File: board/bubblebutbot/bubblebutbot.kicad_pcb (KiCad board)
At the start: 2 copper layers, 66.5 x 28.4 mm, 59 parts, among them J1 JST XH, J10 JST XH, J13 JST XH, J2 USB_C_Receptacle, J3 Conn_01x03_Socket, J4 Conn_01x03_Socket, J7 Conn_01x03_Socket, SW1 SW_Push, SW2 SW_Push, U1 DRV8833PWP, U2 ESP32-S3-WROOM-1, U3 AP63203WU, U4 LIS3DH

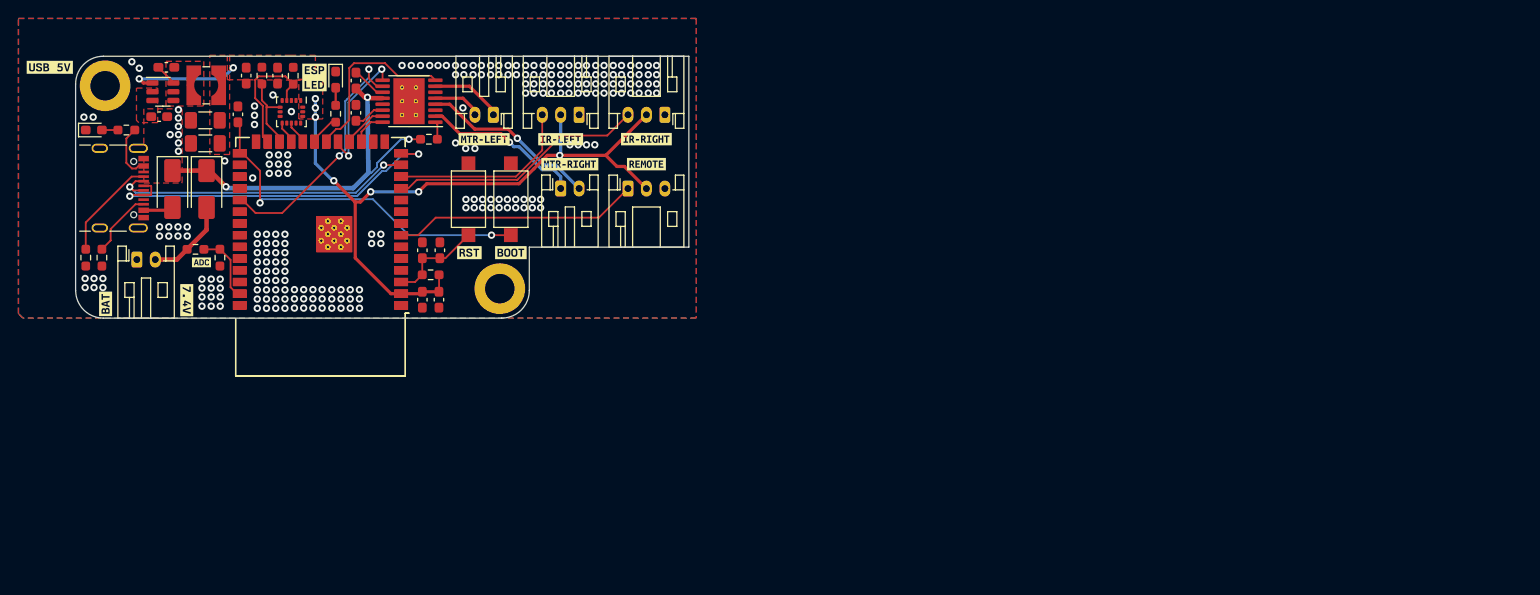
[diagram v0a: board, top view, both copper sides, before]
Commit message: prod 1v7
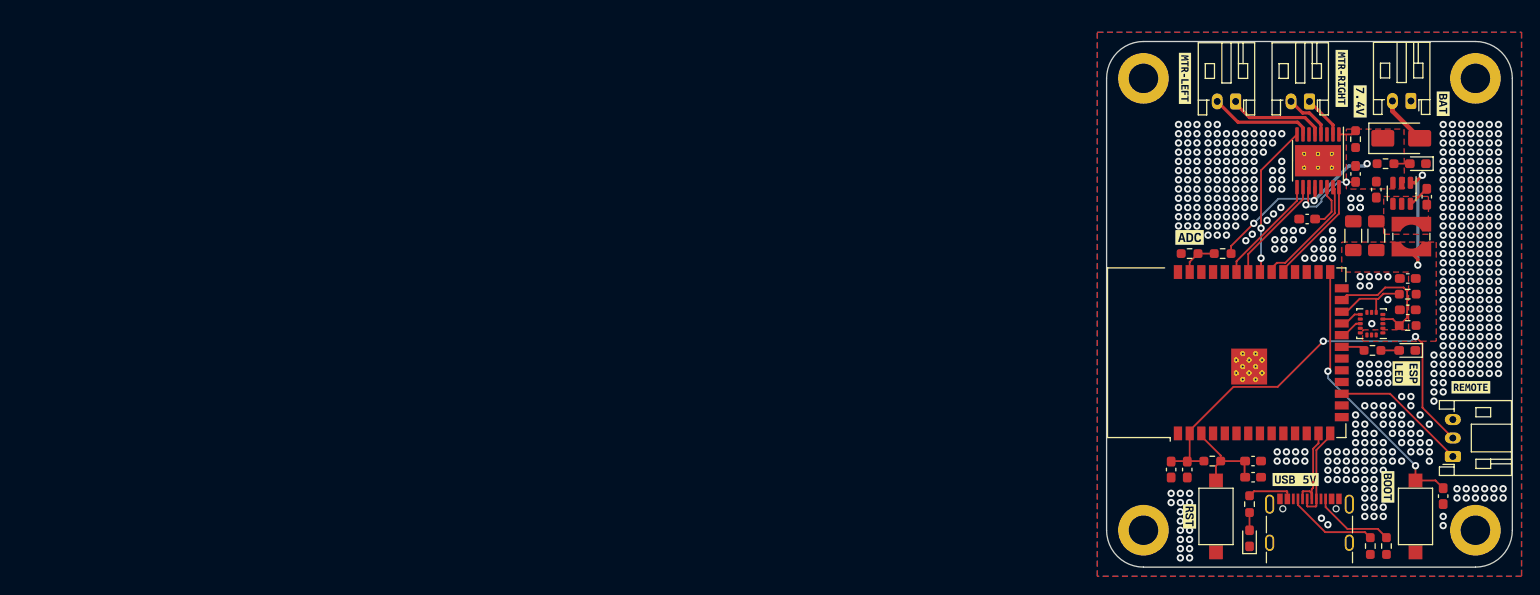
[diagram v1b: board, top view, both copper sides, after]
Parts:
- removed J3, J4: Conn_01x03_Socket, Connector_JST:JST_PH_S3B-PH-K_1x03_P2.00mm_Horizontal
- removed the U2 at (97.8, 47.4)
- removed kibuzzard-656B6BB3: G***, kibuzzard-656B6BB3
- removed kibuzzard-65B534D1: G***, kibuzzard-65B534D1
- removed kibuzzard-65B534EC: G***, kibuzzard-65B534EC
- removed kibuzzard-65B53FA4: G***, kibuzzard-65B53FA4
- added H3: MountingHole, MountingHole:MountingHole_3.2mm_M3_ISO14580_Pad, F.Cu at (223.0, 77.0)
- added H4: MountingHole, MountingHole:MountingHole_3.2mm_M3_ISO14580_Pad, F.Cu at (187.0, 28.0)
- added R3: 5.1K, Resistor_SMD:R_0603_1608Metric_Pad0.98x0.95mm_HandSolder, F.Cu at (213.2, 37.2)
- added kibuzzard-65BE7DA5: G***, kibuzzard-65BE7DA5, F.Cu at (192.0, 45.2)
- added kibuzzard-65BE89A1: G***, kibuzzard-65BE89A1, B.Cu at (205.8, 59.5)
- D2: value SS14 -> LED; footprint Diode_SMD:D_SMA -> LED_SMD:LED_0603_1608Metric_Pad1.05x0.95mm_HandSolder
- moved kibuzzard-65B53096 146.7 mm to (219.5, 30.8), turned to -90 degrees
- moved R4 142.8 mm to (211.6, 78.7)
- moved R7 142.8 mm to (213.3, 78.7)
- moved kibuzzard-65B52192 142.3 mm to (203.5, 71.5)
- moved J1 139.2 mm to (216.0, 30.4), turned to 180 degrees
- moved C11 137.4 mm to (217.7, 40.8), turned to 90 degrees
- moved C14 137.1 mm to (219.5, 73.3), turned to -90 degrees
- moved J2 135.4 mm to (205.0, 77.3), turned to 0 degrees
- moved D2 135.1 mm to (216.8, 37.2), turned to 180 degrees
- moved U3 134.8 mm to (215.0, 40.5), turned to -90 degrees
- moved D3 132.9 mm to (198.5, 77.9), turned to 90 degrees
- moved C9 132.2 mm to (212.2, 40.1), turned to -90 degrees
- moved L1 131.7 mm to (216.1, 45.2), turned to 0 degrees
- moved D4 129.7 mm to (214.9, 34.5), turned to 0 degrees
- moved kibuzzard-65B53DEB 129.1 mm to (210.5, 30.5)
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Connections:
- net MOTOR-RIGHT-FL renamed MOTOR-RIGHT-A
- net MOTOR-RIGHT-FR renamed MOTOR-RIGHT-B
- D2 pad 1: BAT_OUT -> GND
- D2 pad 2: 5V_USB_POWER -> Net-(D2-A)
- J10 pad 1: MOTOR-LEFT-FL -> MOTOR-LEFT-A
- J10 pad 2: MOTOR-LEFT-FR -> MOTOR-LEFT-B
- R6 pad 2: +7.5V -> BAT_OUT
- U1 pad 5: MOTOR-LEFT-FR -> MOTOR-LEFT-A
- U1 pad 7: MOTOR-LEFT-FL -> MOTOR-LEFT-B
- U2 pad 10: ESP32-SRV-F -> unconnected-(U2-GPIO17/U1TXD/ADC2_CH6-Pad10)
- U2 pad 11: ESP32-IR-FR -> unconnected-(U2-GPIO18/U1RXD/ADC2_CH7/CLK_OUT3-Pad11)
- U2 pad 12: ESP32-IR-FL -> unconnected-(U2-GPIO8/TOUCH8/ADC1_CH7/SUBSPICS1-Pad12)
- U2 pad 17: ESP32-MOTOR-AIN1 -> ESP32-REMOTE
- U2 pad 18: ESP32-MOTOR-AIN2 -> unconnected-(U2-GPIO10/TOUCH10/ADC1_CH9/FSPICS0/FSPIIO4/SUBSPICS0-Pad18)
- U2 pad 19: ESP32-MOTOR-BIN1 -> unconnected-(U2-GPIO11/TOUCH11/ADC2_CH0/FSPID/FSPIIO5/SUBSPID-Pad19)
- U2 pad 20: ESP32-MOTOR-FAULT -> unconnected-(U2-GPIO12/TOUCH12/ADC2_CH1/FSPICLK/FSPIIO6/SUBSPICLK-Pad20)
- U2 pad 31: ESP32-MOTOR-BIN2 -> ESP32-MOTOR-AIN1
- U2 pad 32: unconnected-(U2-MTCK/GPIO39/CLK_OUT3/SUBSPICS1-Pad32) -> ESP32-MOTOR-AIN2
- U2 pad 33: unconnected-(U2-MTDO/GPIO40/CLK_OUT2-Pad33) -> ESP32-MOTOR-FAULT
- U2 pad 34: unconnected-(U2-MTDI/GPIO41/CLK_OUT1-Pad34) -> ESP32-MOTOR-BIN2
- U2 pad 35: unconnected-(U2-MTMS/GPIO42-Pad35) -> ESP32-MOTOR-BIN1
- U2 pad 5: ESP32-LF-RIGHT -> unconnected-(U2-GPIO5/TOUCH5/ADC1_CH4-Pad5)
- U2 pad 6: ESP32-LF-LEFT -> unconnected-(U2-GPIO6/TOUCH6/ADC1_CH5-Pad6)
- U2 pad 7: ESP32-REMOTE -> unconnected-(U2-GPIO7/TOUCH7/ADC1_CH6-Pad7)
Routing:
- net ESP32-D+: track 39.3 -> 10.3 mm, vias 2 -> 0
- net +3.3V: track 89.9 -> 61.2 mm, vias 9 -> 4
- net ESP32-IR-FR: track 27.9 -> 0.00 mm
- net ESP32-D-: track 34.3 -> 9.89 mm, vias 2 -> 0
- net BAT_OUT: track 41.7 -> 20.9 mm
- net ESP32-IR-FL: track 20.3 -> 0.00 mm
- net ESP32-MOTOR-BIN2: track 27.5 -> 11.7 mm, vias 2 -> 0
- net MOTOR-RIGHT-B: track 19.4 -> 5.36 mm, vias 1 -> 0
- net MOTOR-RIGHT-A: track 17.6 -> 4.63 mm, vias 1 -> 0
- net ESP32-REMOTE: track 26.7 -> 14.9 mm
- net MOTOR-LEFT-B: track 0.00 -> 11.2 mm
- net MOTOR-LEFT-A: track 0.00 -> 10.7 mm
- net ESP32-BOOT0: track 38.8 -> 30.0 mm
- net ESP32-MOTOR-AIN1: track 3.80 -> 11.7 mm
- net MOTOR-LEFT-FL: track 7.86 -> 0.00 mm
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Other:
- board size 66.5 x 28.4 mm -> 44 x 57 mm
- board text added: "locked"
- board text removed: "a) Search for the {dblquote}BattleButBot{dblquote} Wi-Fi network b) Connect c) Open your browser d) Type {dblquote}bot.local{dblquote} as the URL e) ? f) Enjoy :)"
